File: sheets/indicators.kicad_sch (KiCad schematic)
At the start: 18 parts, among them Q3 AO3400A

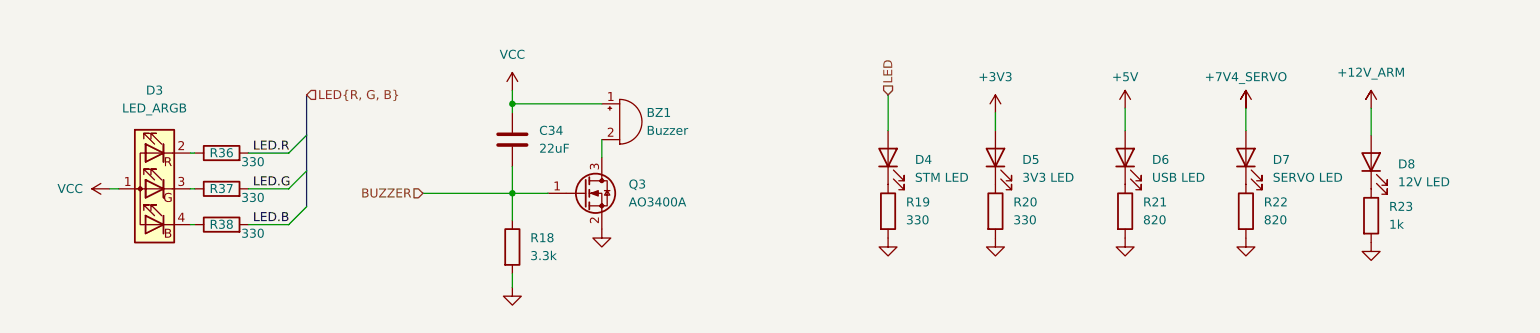
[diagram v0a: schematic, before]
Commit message: Rev1 schematic done
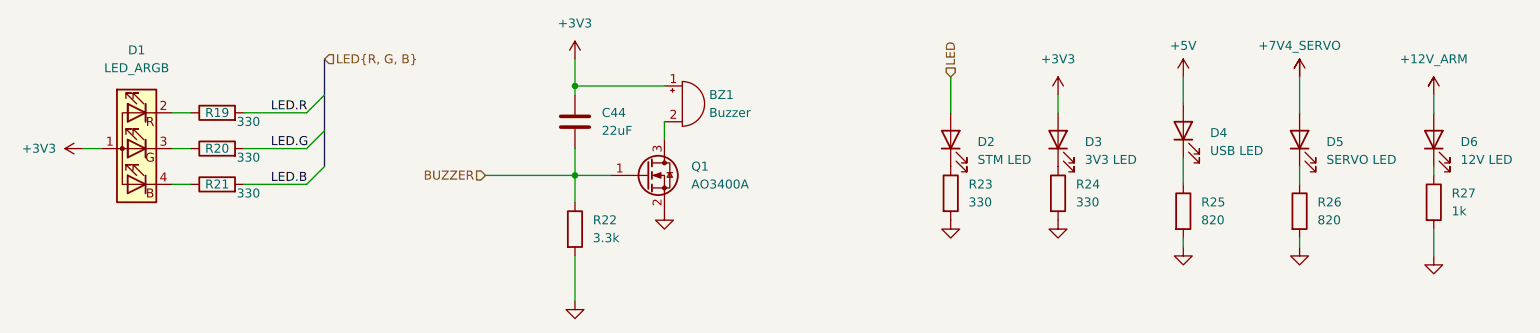
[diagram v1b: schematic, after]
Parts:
- renumbered C34 to C44, D3 to D1, D4 to D2, D5 to D3, D6 to D4, D7 to D5, D8 to D6, Q3 to Q1, R36 to R19, R37 to R20, R38 to R21, R18 to R22, R19 to R23, R20 to R24, R21 to R25, R22 to R26, R23 to R27
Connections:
- net VCC is gone; now on net +3V3: BZ1.1 (+), C44.1, D1.1 (A)
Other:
- moved on the sheet: BZ1, C44, D1, D2, D3, D4, D5, D6, Q1, R19, R20, R21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
